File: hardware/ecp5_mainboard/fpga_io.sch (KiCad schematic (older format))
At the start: 76 parts, among them J10 UART, J11 FLASH, J12 JTAG, J5 EXT0, J6 EXT1, J7 EXT2, J9 PMOD_01, Q9 BSH111BKR, SW6 SW_Push, U15 ECP5UM5G_85_CABGA756, U26 XL_XO_LVDS, U27 W25Q

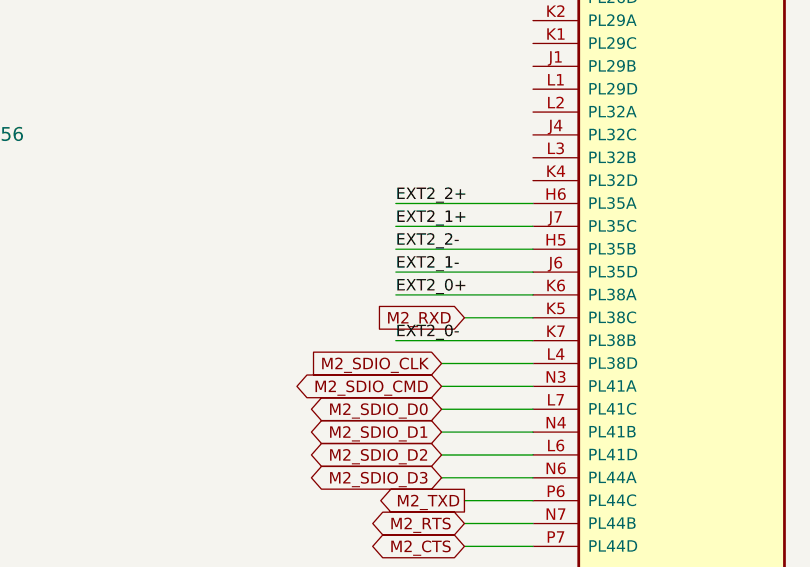
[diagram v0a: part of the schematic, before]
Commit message: hardware/mainboard: Misc routing
Signed-off-by: David Shah <davey1576@gmail.com>
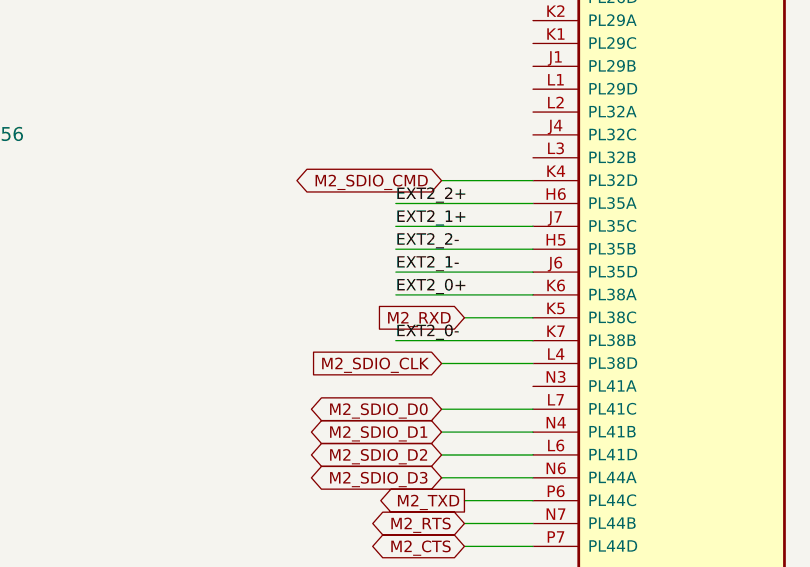
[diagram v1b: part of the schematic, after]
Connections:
- net M2_SDIO_CMD: now also U15.K4 (PL32D); no longer U15.N3 (PL41A)
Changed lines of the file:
@@
 Text GLabel 12150 13200 0    50   Input ~ 0
 M2_SDIO_CLK
-Text GLabel 12150 13300 0    50   BiDi ~ 0
+Text GLabel 12150 12400 0    50   BiDi ~ 0
 M2_SDIO_CMD
 Text GLabel 12150 13400 0    50   BiDi ~ 0
@@
 	12150 13200 12550 13200
 Wire Wire Line
-	12150 13300 12550 13300
+	12150 12400 12550 12400
 Wire Wire Line
 	12150 13400 12550 13400
